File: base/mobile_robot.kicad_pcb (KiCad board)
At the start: 2 copper layers, 85.6 x 49 mm, 74 parts, among them J1 USB_B_Micro, J2 Conn_02x05_Odd_Even, J3 Motor Power, J4 Conn_01x06, J5 Conn_01x06, Q1 BSS138, Q2 BSS138, Q3 BSS138, Q4 BSS138, SW1 SW_SPDT, U1 AMS1117-3.3, U2 STM32F103C8T6, U3 MPU-6050, U4 L298HN, U5 OP07, U6 OP07, Y1 16M

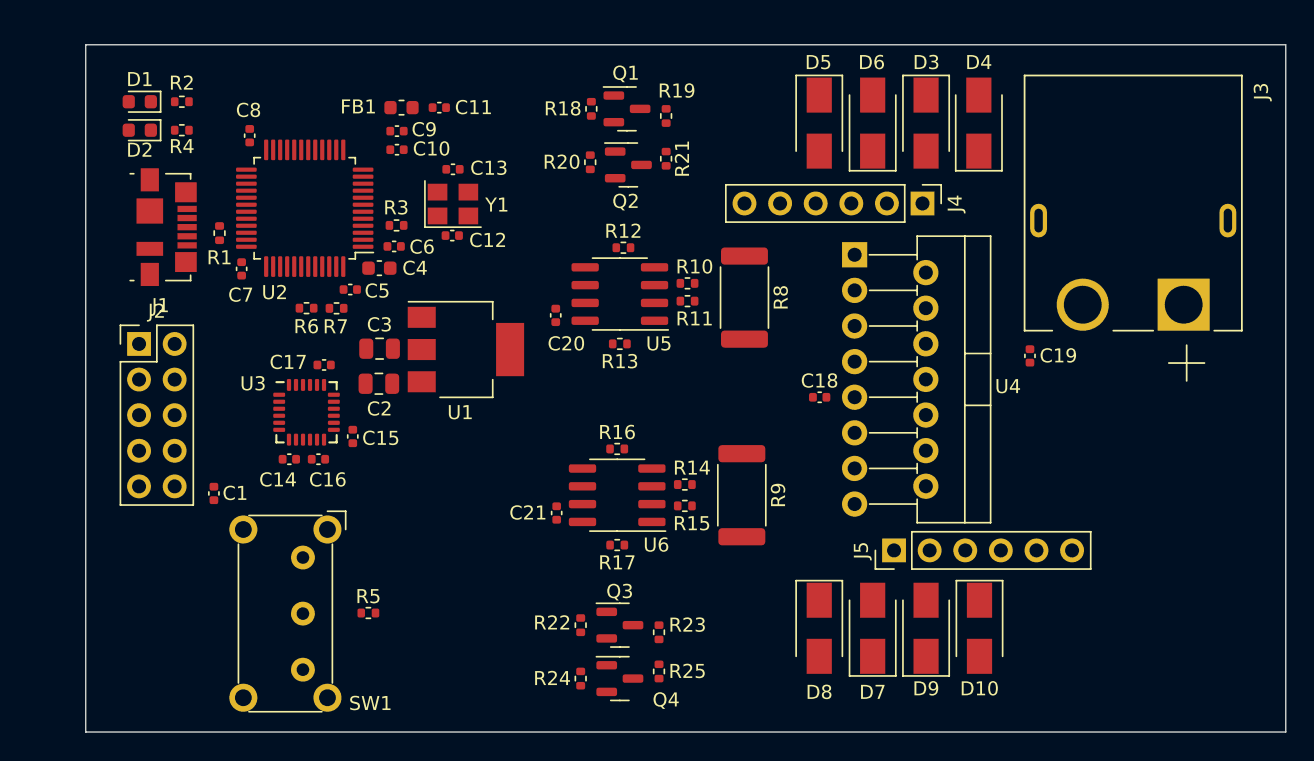
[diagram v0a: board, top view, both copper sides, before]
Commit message: Pretty much finished pcb layout and routing
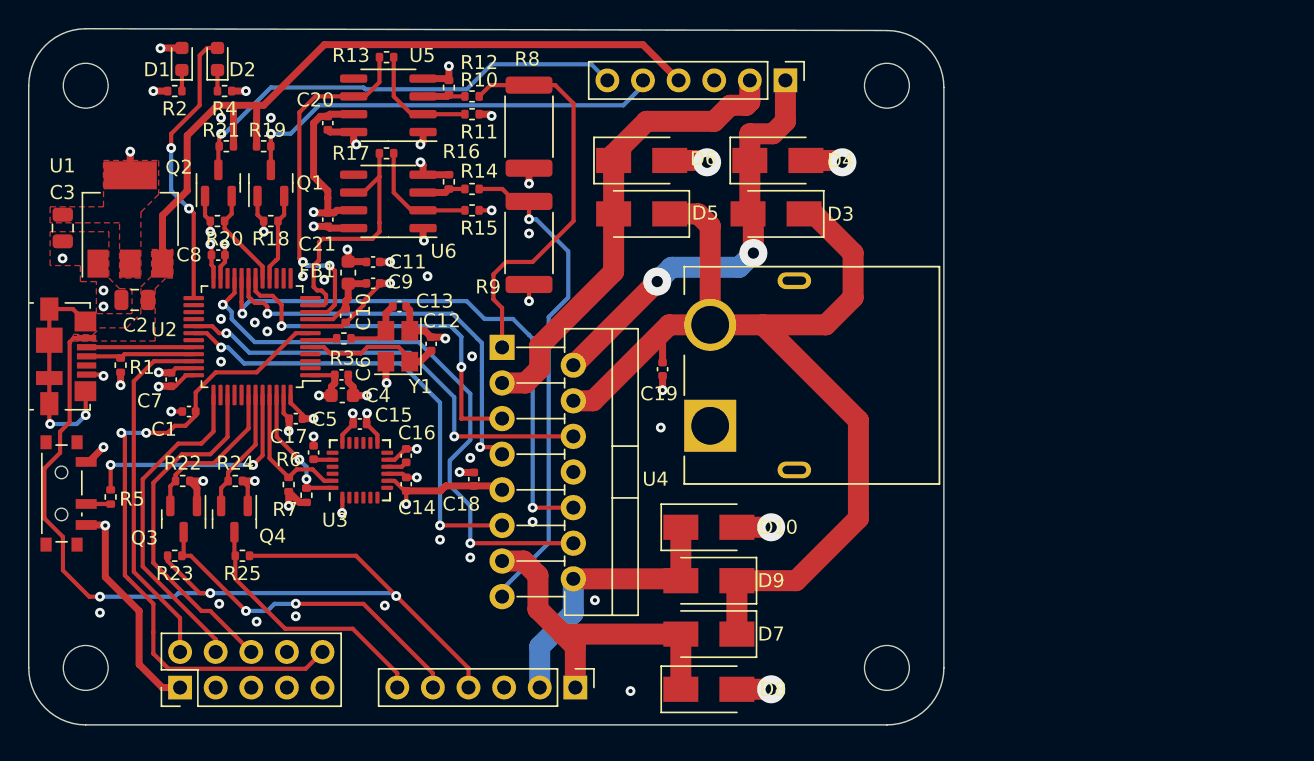
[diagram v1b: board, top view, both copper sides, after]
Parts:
- added H1: MountingHole, MountingHole:MountingHole_3.2mm_M3, F.Cu at (25.4, 28.3)
- added H2: MountingHole, MountingHole:MountingHole_3.2mm_M3, F.Cu at (82.5, 28.3)
- added H3: MountingHole, MountingHole:MountingHole_3.2mm_M3, F.Cu at (25.4, 69.8)
- added H4: MountingHole, MountingHole:MountingHole_3.2mm_M3, F.Cu at (82.5, 69.8)
- SW1: footprint Button_Switch_THT:SW_E-Switch_EG1224_SPDT_Angled -> Button_Switch_SMD:SW_SPDT_PCM12
- moved R23 35.0 mm to (31.8, 61.8), turned to 0 degrees
- moved R17 32.4 mm to (46.9, 33.1)
- moved Q3 32.0 mm to (32.4, 59.2), turned to -90 degrees
- moved R21 31.4 mm to (35.4, 32.6), turned to 180 degrees
- moved R25 30.8 mm to (36.6, 61.8), turned to 180 degrees
- moved R22 30.2 mm to (32.3, 56.5), turned to 180 degrees
- moved Q4 29.8 mm to (36.0, 59.2), turned to -90 degrees
- moved Q2 29.3 mm to (34.9, 35.3), turned to 90 degrees
- moved R19 28.8 mm to (38.1, 32.6), turned to 0 degrees
- moved R24 28.4 mm to (36.1, 56.5), turned to 180 degrees
- moved R20 26.9 mm to (34.8, 38.0), turned to 0 degrees
- moved J3 26.6 mm to (75.9, 49.0), turned to -90 degrees
- moved U6 26.6 mm to (47.0, 36.6)
- moved C21 26.5 mm to (42.7, 37.9)
- moved R13 26.4 mm to (46.9, 26.3)
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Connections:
- U2 pad 3: HSE_IN -> unconnected-(U2-Pad3)
- U2 pad 4: HSE_OUT -> unconnected-(U2-Pad4)
- U2 pad 5: unconnected-(U2-Pad5) -> HSE_IN
- U2 pad 6: unconnected-(U2-Pad6) -> HSE_OUT
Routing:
- net V_ENC: track 0.00 -> 122.9 mm, vias 0 -> 3
- net +12V: track 0.00 -> 75.0 mm
- net +3V3: track 0.00 -> 73.4 mm, vias 0 -> 17
- net GND: track 0.00 -> 69.1 mm, vias 0 -> 60
- net NRST: track 0.00 -> 47.1 mm, vias 0 -> 2
- net MB_IN2: track 0.00 -> 42.0 mm, vias 0 -> 2
- net MB_IN1: track 0.00 -> 39.9 mm, vias 0 -> 2
- net MB_RS: track 0.00 -> 35.5 mm, vias 0 -> 1
- net MA_OUT2: track 0.00 -> 33.4 mm
- net /MA_ENC_CH2_RAW: track 0.00 -> 32.8 mm, vias 0 -> 1
- net MB_EN: track 0.00 -> 32.8 mm, vias 0 -> 2
- net MA_EN: track 0.00 -> 32.0 mm, vias 0 -> 2
- net /MA_ENC_CH1_RAW: track 0.00 -> 30.9 mm, vias 0 -> 1
- net MA_OUT1: track 0.00 -> 30.7 mm, vias 0 -> 2
- net MA_IN2: track 0.00 -> 28.9 mm, vias 0 -> 2
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- added copper zone on F.Cu, net +3V3
- added copper zone on In2.Cu, net +3V3
- added copper zone on F.Cu, net GND
- added copper zone on In1.Cu, net GND
- added copper zone on In2.Cu, net GND
- added copper zone on F.Cu, net V_ENC
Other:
- board size 85.6 x 49 mm -> 65.3 x 49.7 mm
- copper layers 2 -> 4
